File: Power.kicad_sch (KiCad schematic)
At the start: 41 parts, among them J7 POWER, U10 74HC32, U11 74HC14, U12 74HC00, U4 74HC32, U6 74HC32, U7 74HC00, U9 74HC04

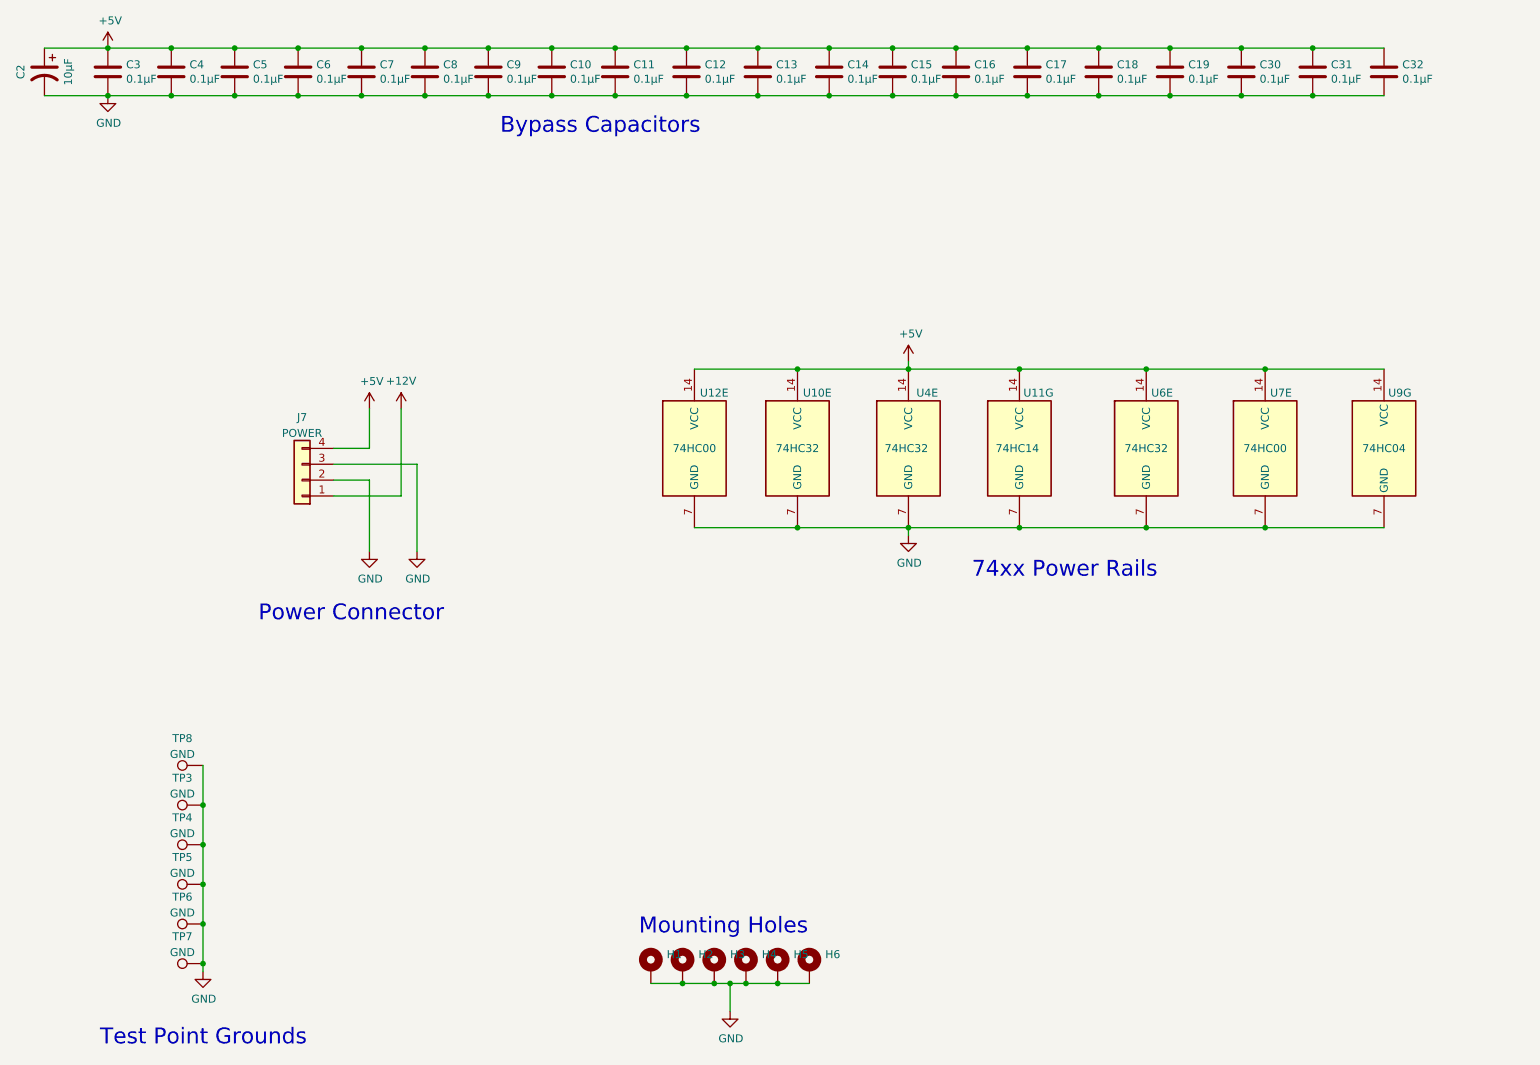
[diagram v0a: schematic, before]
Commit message: Schematic cleanup
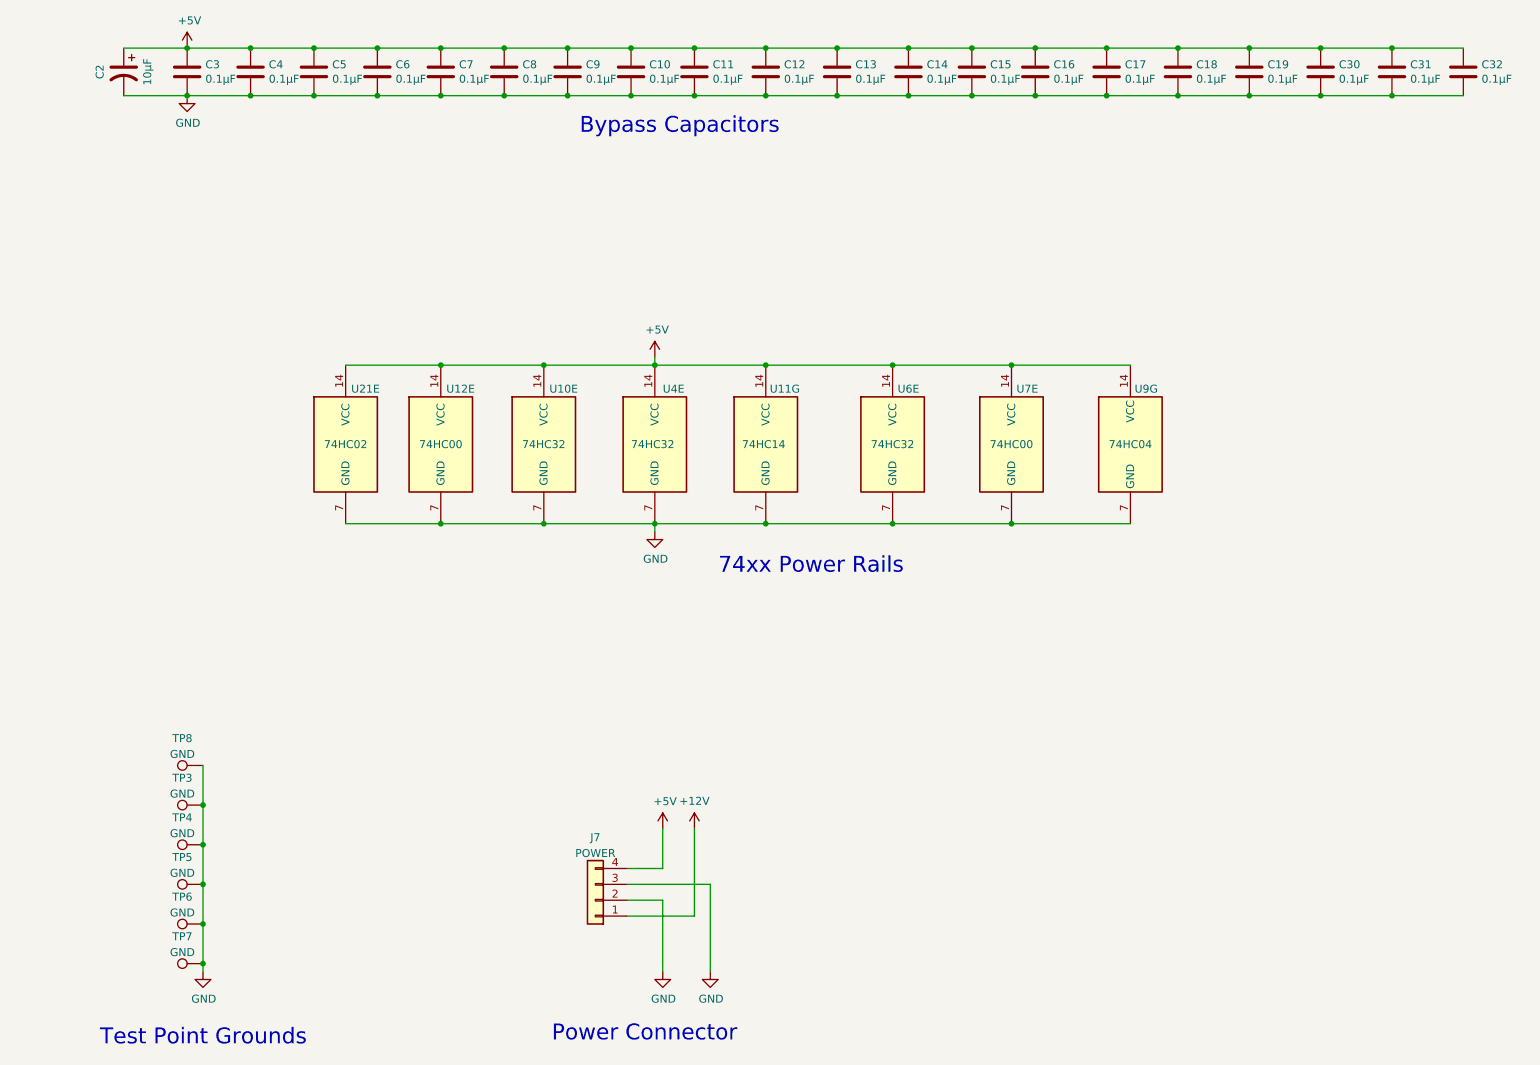
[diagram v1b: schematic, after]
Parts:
- removed H1, H2, H3, H4, H5, H6: MountingHole_Pad, MountingHole:MountingHole_3.2mm_M3_Pad_Via, symbol Mechanical:MountingHole_Pad
- added U21: 74HC02, Package_DIP:DIP-14_W7.62mm_LongPads, symbol 74xx:74HC02
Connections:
- net +5V: now also U21.14 (VCC)
- net GND: now also U21.7 (GND)
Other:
- note removed: "Mounting Holes"
- moved on the sheet: C10, C11, C12, C13, C14, C15, C16, C17, C18, C19, C2, C3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
